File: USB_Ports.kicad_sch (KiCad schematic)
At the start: 28 parts, among them IC2 TPS2066TDGNRQ1, IC3 TPS2066TDGNRQ1, J10 3-2172091-2, J5 3-2172091-2, J6 3-2172091-2, J8 3-2172091-2

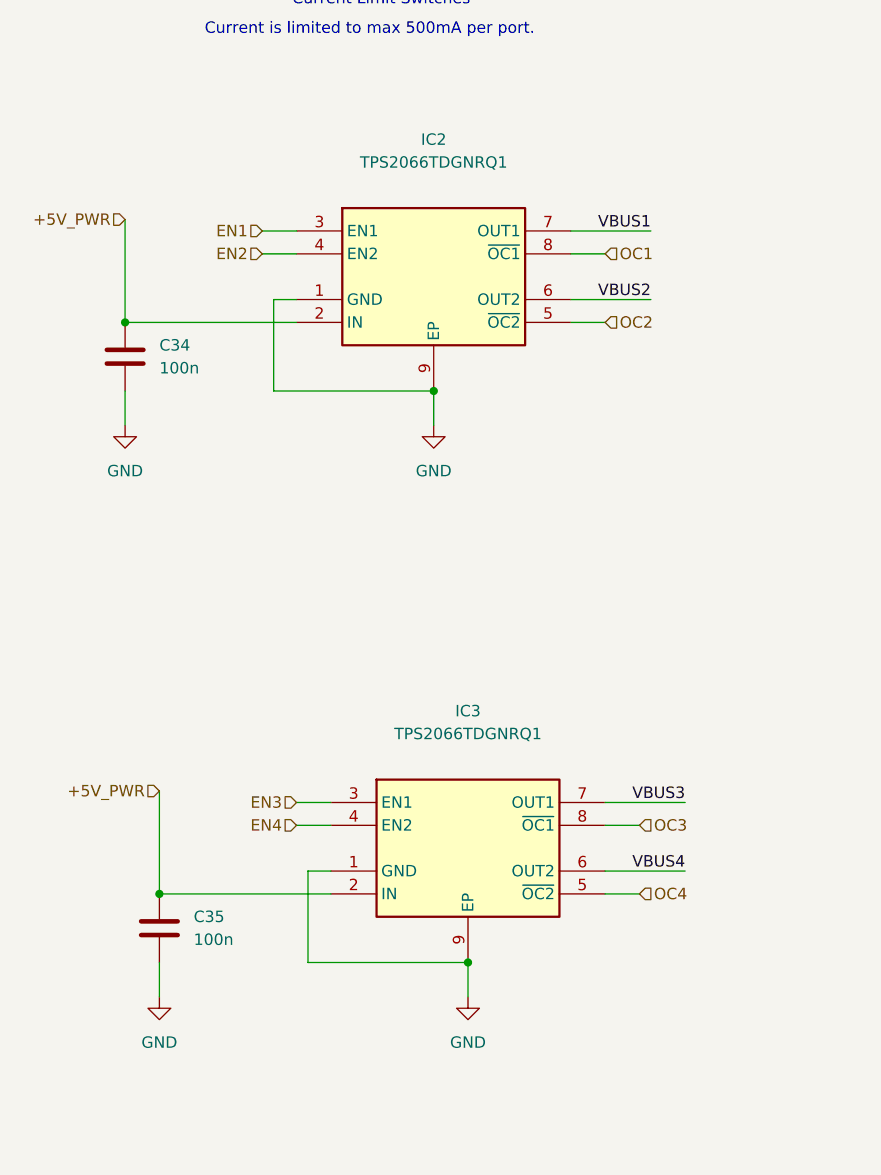
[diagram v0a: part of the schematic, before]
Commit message: think im done with schematic
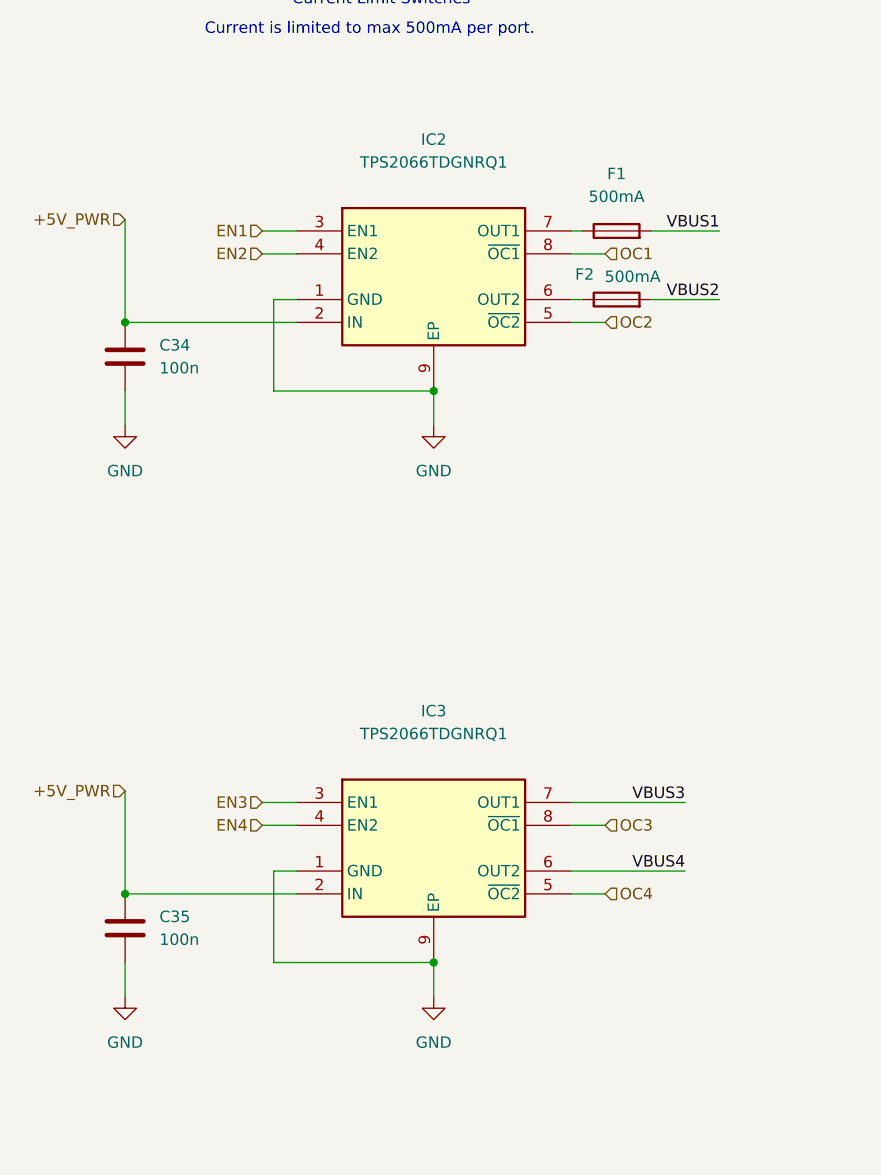
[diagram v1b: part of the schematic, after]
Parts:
- added F1, F2: 500mA, symbol Device:Fuse
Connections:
- net VBUS1: now also F1.2; no longer IC2.7 (OUT1)
- net VBUS2: now also F2.2; no longer IC2.6 (OUT2)
- new net: F2.1, IC2.6 (OUT2)
- new net: F1.1, IC2.7 (OUT1)
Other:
- moved on the sheet: C35, IC3
